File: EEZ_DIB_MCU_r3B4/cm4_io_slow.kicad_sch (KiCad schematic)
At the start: 6 parts, among them J3 HR911130A

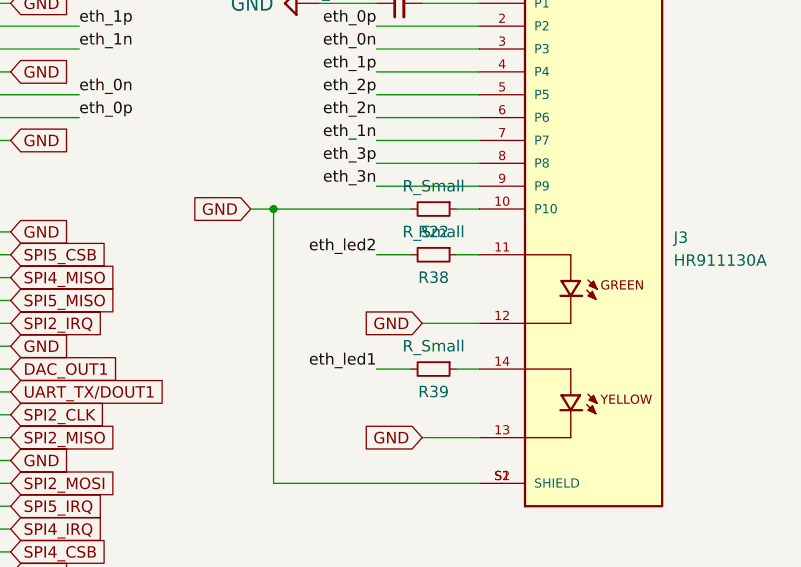
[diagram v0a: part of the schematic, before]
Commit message: Adding DSI connector
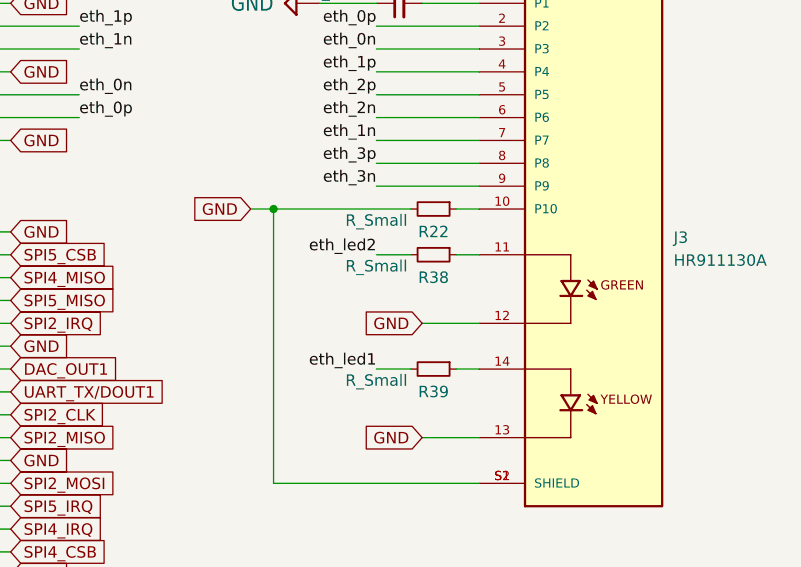
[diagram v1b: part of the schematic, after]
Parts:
- C26: footprint (none) -> Capacitor_SMD:C_0603_1608Metric
- R22, R38, R39: footprint (none) -> Resistor_SMD:R_0603_1608Metric
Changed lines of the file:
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@@
       (effects (font (size 1.27 1.27)))
     )
-    (property "Value" "R_Small" (at 212.09 105.41 90)
-      (effects (font (size 1.27 1.27)))
-    )
-    (property "Footprint" "" (at 212.09 107.95 0)
+    (property "Value" "R_Small" (at 205.74 109.22 90)
+      (effects (font (size 1.27 1.27)))
+    )
+    (property "Footprint" "Resistor_SMD:R_0603_1608Metric" (at 212.09 107.95 0)
       (effects (font (size 1.27 1.27)) hide)
     )
@@
       (effects (font (size 1.27 1.27)))
     )
-    (property "Footprint" "" (at 208.28 80.01 0)
+    (property "Footprint" "Capacitor_SMD:C_0603_1608Metric" (at 208.28 80.01 0)
       (effects (font (size 1.27 1.27)) hide)
     )
@@
       (effects (font (size 1.27 1.27)))
     )
-    (property "Value" "R_Small" (at 212.09 118.11 90)
-      (effects (font (size 1.27 1.27)))
-    )
-    (property "Footprint" "" (at 212.09 120.65 0)
+    (property "Value" "R_Small" (at 205.74 121.92 90)
+      (effects (font (size 1.27 1.27)))
+    )
+    (property "Footprint" "Resistor_SMD:R_0603_1608Metric" (at 212.09 120.65 0)
       (effects (font (size 1.27 1.27)) hide)
     )
@@
       (effects (font (size 1.27 1.27)))
     )
-    (property "Value" "R_Small" (at 212.09 100.33 90)
-      (effects (font (size 1.27 1.27)))
-    )
-    (property "Footprint" "" (at 212.09 102.87 0)
-      (effects (font (size 1.27 1.27)) hide)
-    )
+    (property "Value" "R_Small" (at 205.74 104.14 90)
+      (effects (font (size 1.27 1.27)))
+    )
+    (property "Footprint" "Resistor_SMD:R_0603_1608Metric" (at 212.09 102.87 0)
+      (effects (font (size 1.27 1.27)) hide)
+    )
